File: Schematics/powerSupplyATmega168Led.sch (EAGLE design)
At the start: 4 parts, among them IC1 LM2931T

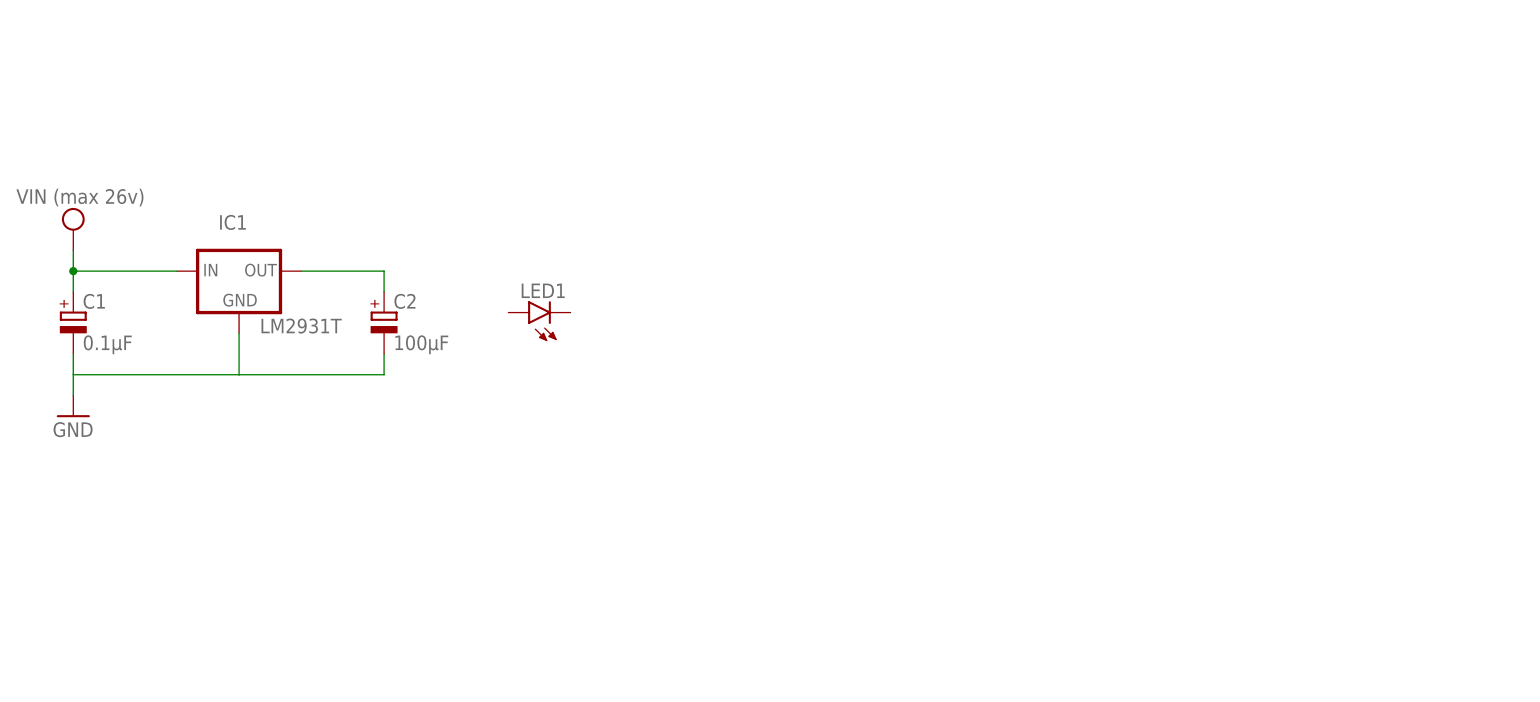
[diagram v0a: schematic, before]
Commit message: Added different schematics and code
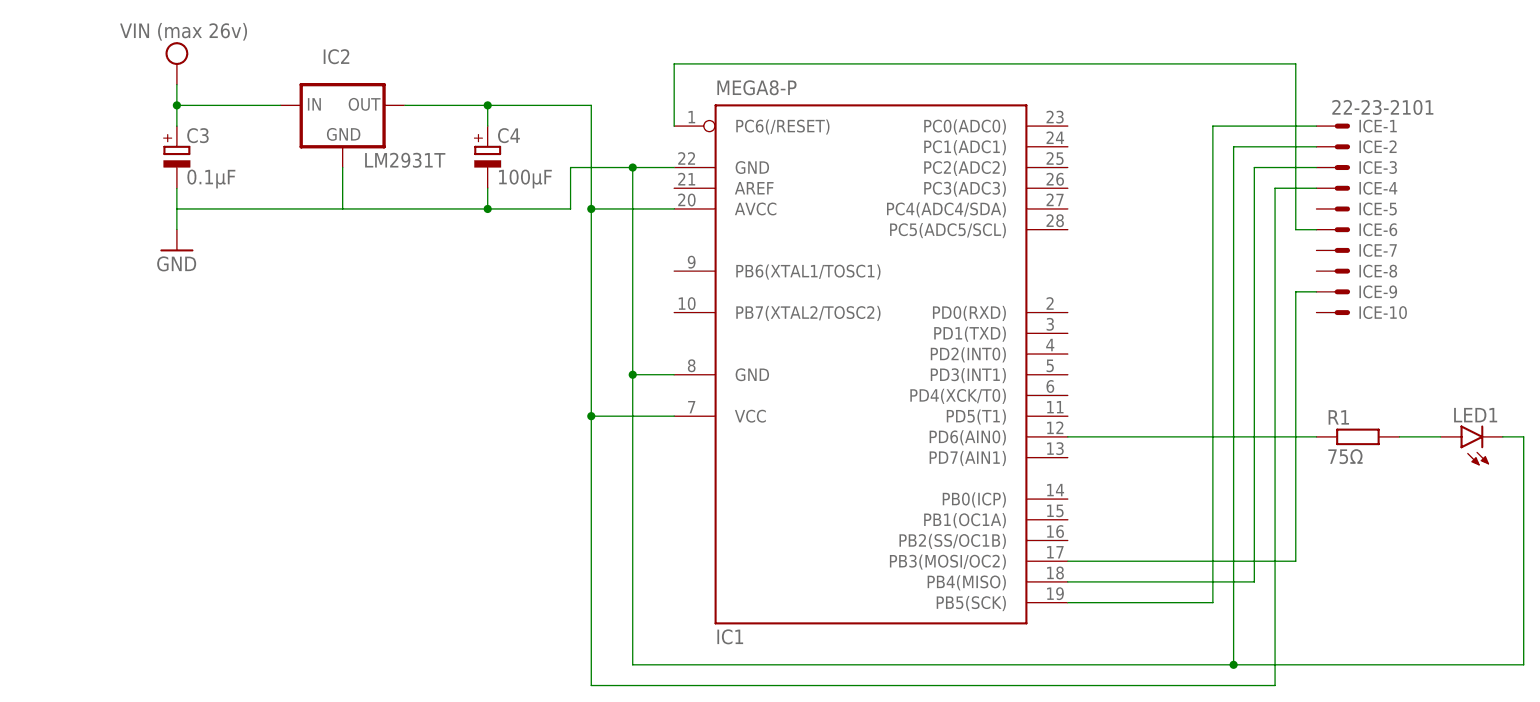
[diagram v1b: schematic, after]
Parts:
- removed C1: 0.1µF, rcl:CPOL-EUE5-5
- removed C2: 100µF, rcl:CPOL-EUE5-5
- added C3: 0.1µF, rcl:CPOL-EUE5-5
- added C4: 100µF, rcl:CPOL-EUE5-5
- added IC2: LM2931T, v-reg-3:LM2931T
- added ICE: 22-23-2101, con-molex:22-23-2101
- added R1: 75Ω, rcl:R-EU_0617/17
- IC1: value LM2931T -> MEGA8-P; device v-reg-3:LM2931T -> atmel:MEGA8-P
- LED1: value (none) -> SFH482; device led:LED5MM -> led:SFH482
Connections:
- new net N$2: IC1.PB5(SCK), ICE-1.S
- new net N$3: IC1.PB4(MISO), ICE-3.S
- new net N$4: C4.+, IC1.AVCC, IC1.VCC@1, IC2.OUT, ICE-4.S
- new net N$5: IC1.PC6(/RESET), ICE-6.S
- new net N$6: IC1.PB3(MOSI/OC2), ICE-9.S
- new net N$7: IC1.PD6(AIN0), R1.1
- net GND: now also C3.-, C4.-, IC1.GND@1, IC2.GND, ICE-2.S, LED1.C; no longer C1.-, C2.-
- net N$1: now also LED1.A, R1.2; no longer C2.+, IC1.OUT
- net VCC: now also C3.+, IC2.IN; no longer C1.+, IC1.IN
